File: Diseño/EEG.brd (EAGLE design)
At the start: 49.8 x 80 mm, 38 parts, among them IC2 MCP73831T-2ACI_OT, IC3 LP38692MP-3.3_NOPB, J1 USB3500-30-A-KIT, J2 SJ-3523-SMT-TR, J3 1769

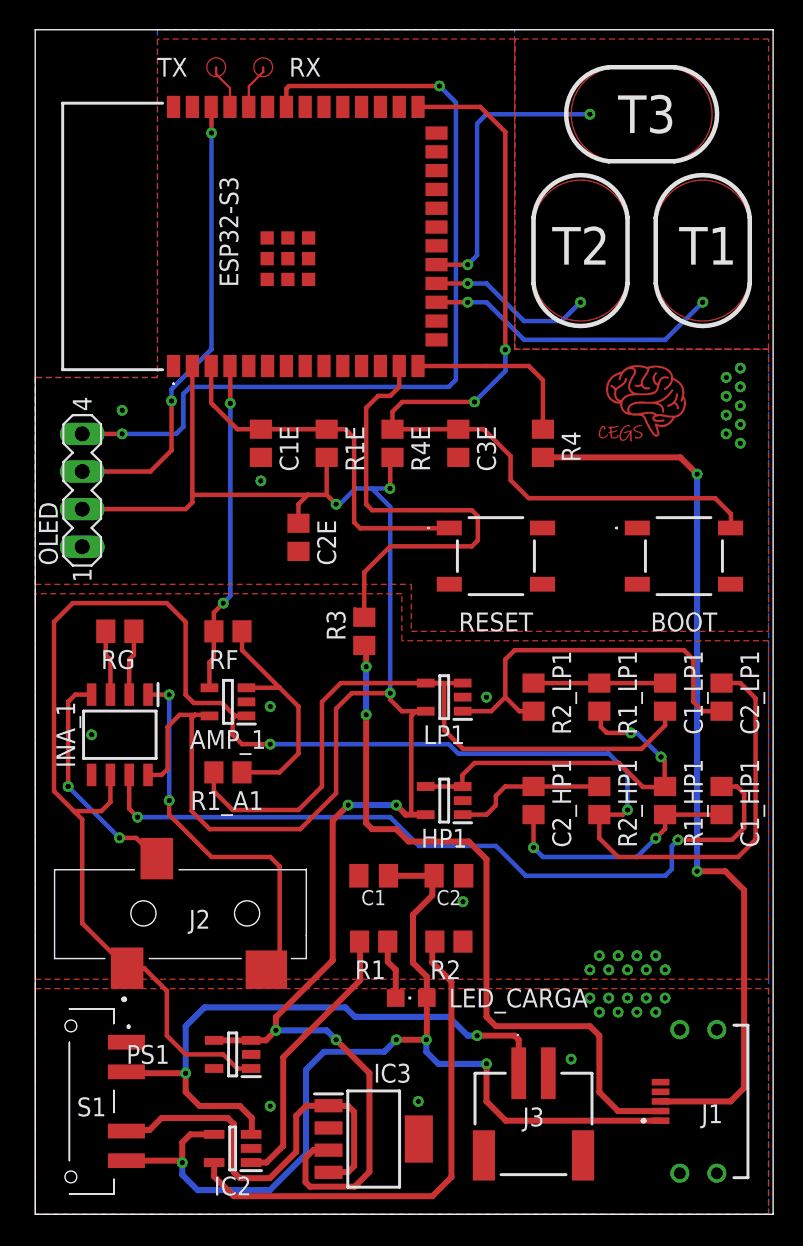
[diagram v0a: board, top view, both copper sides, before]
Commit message: por fin acabamos esto
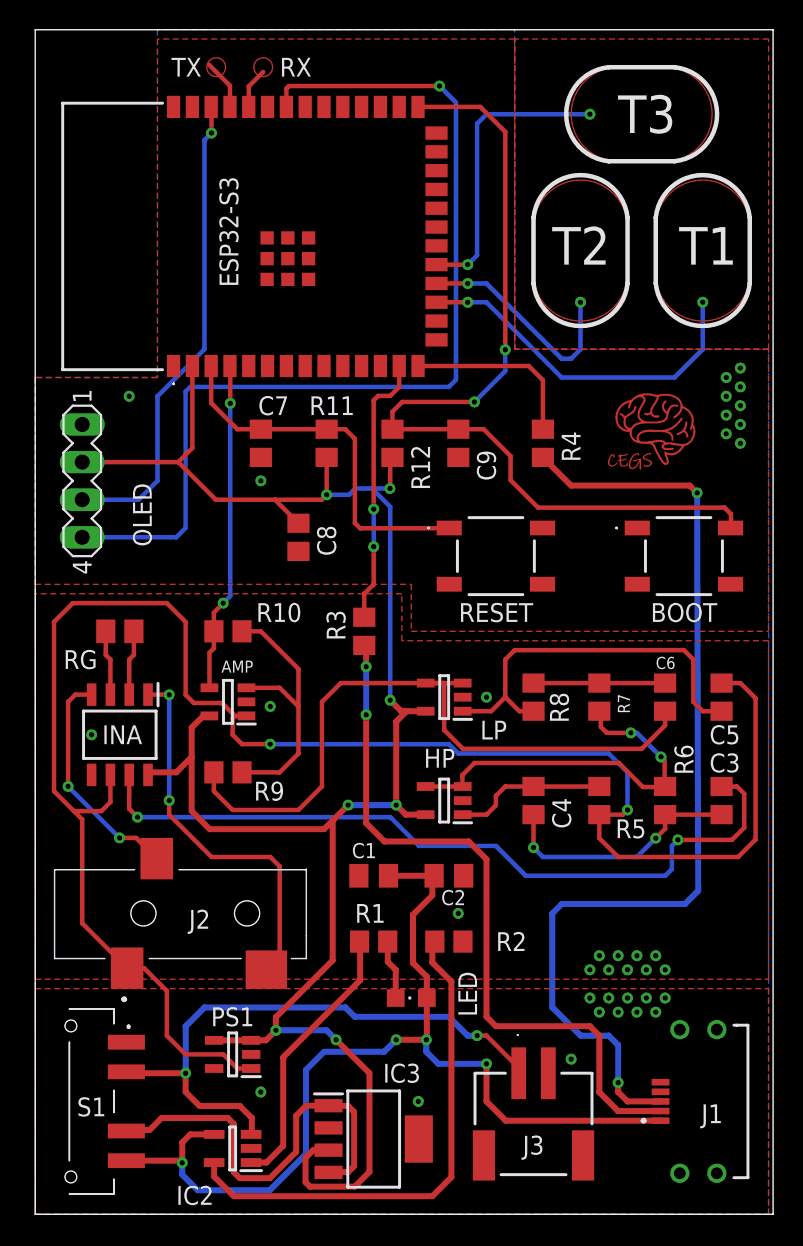
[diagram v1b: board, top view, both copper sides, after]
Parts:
- C1, C2: value (none) -> 10u
- moved OLED 0.63 mm to (3.17, 49.5), turned to 270 degrees
- renumbered AMP_1 to AMP, C1E to C7, C1_HP1 to C3, C1_LP1 to C6, C2E to C8, C2_HP1 to C4, C2_LP1 to C5, C3E to C9, HP1 to HP, INA_1 to INA, LED_CARGA to LED, LP1 to LP, R1E to R11, R1_A1 to R9, R1_HP1 to R6, R1_LP1 to R7, R2_HP1 to R5, R2_LP1 to R8, R4E to R12, RF to R10
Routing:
- net +3V3: track 149.6 -> 130.7 mm
- net N$18: track 32.7 -> 18.4 mm, vias 0 -> 2
- net SDA: track 60.0 -> 67.0 mm, vias 2 -> 1
- net USB_3: track 60.8 -> 66.9 mm
- net TOUCHP_2: track 11.3 -> 15.3 mm
- net TOUCHP_1: track 20.1 -> 24.0 mm
- net N$8: track 16.4 -> 19.0 mm
- net SCL: track 30.9 -> 32.4 mm, vias 2 -> 1
- net +BATT: track 41.0 -> 39.9 mm
- net O4: track 23.0 -> 22.3 mm
- net N$11: track 29.1 -> 28.5 mm
